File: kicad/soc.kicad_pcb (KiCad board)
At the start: 2 copper layers, 104.1 x 63.5 mm, 10 parts, among them J1 JACK_TRS_3PINS, J2 PS/2 Keyboard, J3 PS/2 Mouse, P1 LED MATRIX, P10 CODEC right, P11 CODEC inputs, P2 ALTERA_DE1_GPIO, P9 CODEC left, U2 DS3234

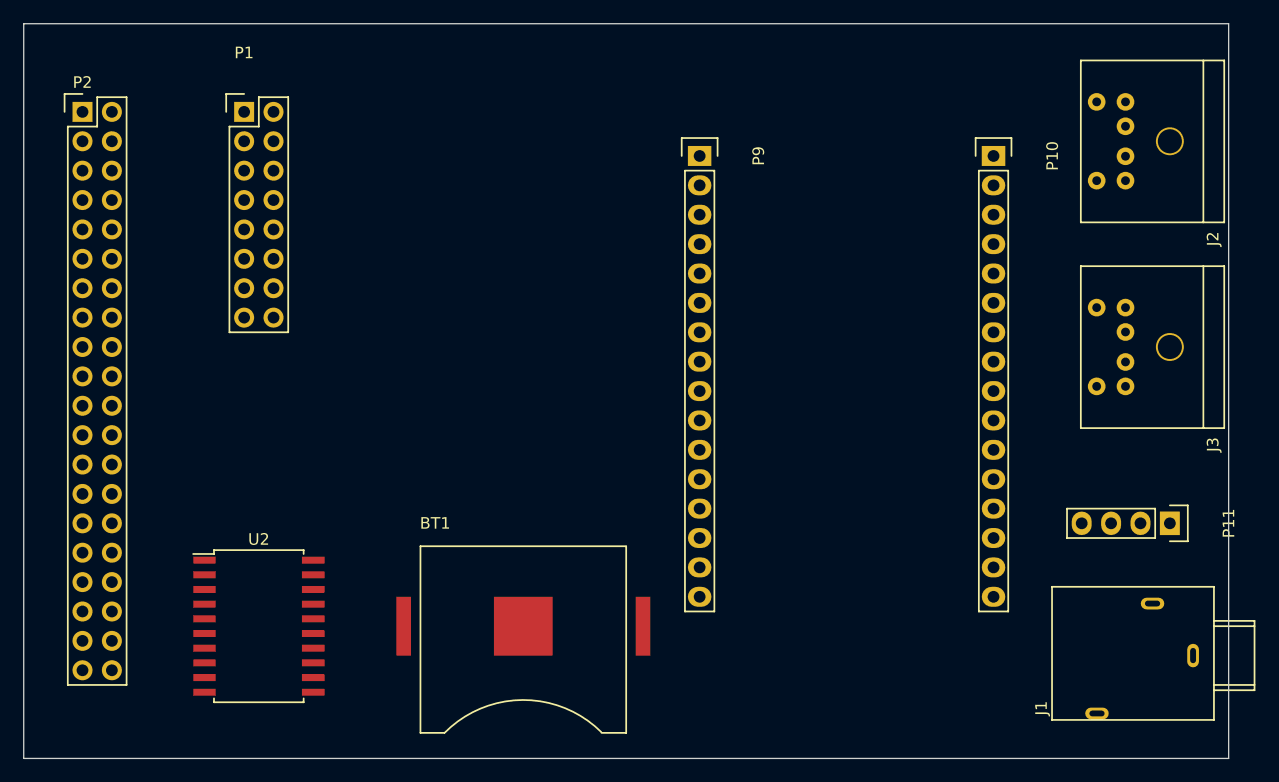
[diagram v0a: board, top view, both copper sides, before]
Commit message: close to final
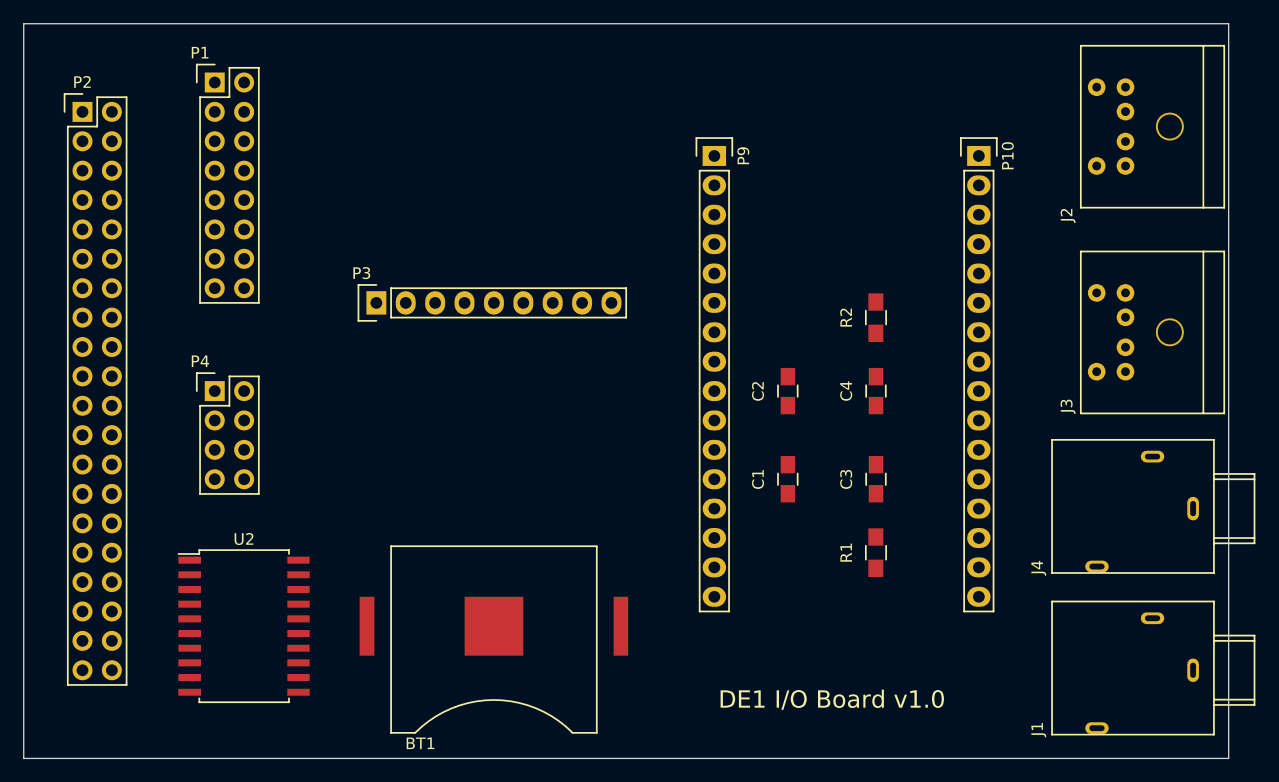
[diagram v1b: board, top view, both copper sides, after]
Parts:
- removed P11: CODEC inputs, Pin_Headers:Pin_Header_Straight_1x04
- added C1: 10nF, Capacitors_SMD:C_0805_HandSoldering, F.Cu at (106.7, 100.3)
- added C2: 10nF, Capacitors_SMD:C_0805_HandSoldering, F.Cu at (106.7, 92.7)
- added C3: 1uF, Capacitors_SMD:C_0805_HandSoldering, F.Cu at (114.3, 100.3)
- added C4: 1uF, Capacitors_SMD:C_0805_HandSoldering, F.Cu at (114.3, 92.7)
- added J4: Line In, mstock-pretty:SJI-3513N, F.Cu at (143.5, 102.9)
- added P3: Bluetooth, Socket_Strips:Socket_Strip_Straight_1x09, F.Cu at (71.1, 85.1)
- added P4: CONN_01X08, Pin_Headers:Pin_Header_Straight_2x04, F.Cu at (57.1, 92.7)
- added R1: 470, Resistors_SMD:R_0805_HandSoldering, F.Cu at (114.3, 106.7)
- added R2: 470, Resistors_SMD:R_0805_HandSoldering, F.Cu at (114.3, 86.4)
- J1: value JACK_TRS_3PINS -> Line Out
- moved P1 3.59 mm to (57.1, 66.0)
- moved BT1 2.54 mm to (81.3, 113.0)
- moved J1 1.27 mm to (143.5, 116.8)
- moved J2 1.27 mm to (139.7, 69.8)
- moved J3 1.27 mm to (139.7, 87.6)
- moved U2 1.27 mm to (59.7, 113.0)
- moved P10 1.27 mm to (123.2, 72.4)
- moved P9 1.27 mm to (100.3, 72.4)
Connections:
- net Net-(J1-Pad2) renamed /L_OUT
- net Net-(J1-Pad3) renamed /R_OUT
- J1 pad 1: Net-(J1-Pad1) -> GNDA
- J2 pad 2: (no net) -> Net-(J2-Pad2)
- J2 pad 6: (no net) -> Net-(J2-Pad6)
- J3 pad 2: (no net) -> Net-(J3-Pad2)
- J3 pad 6: (no net) -> Net-(J3-Pad6)
- P1 pad 12: (no net) -> Net-(P1-Pad12)
- P10 pad 1: (no net) -> Net-(P10-Pad1)
- P10 pad 10: (no net) -> Net-(P10-Pad10)
- P10 pad 11: (no net) -> Net-(P10-Pad11)
- P10 pad 12: (no net) -> Net-(P10-Pad12)
- P10 pad 13: Net-(P10-Pad13) -> GNDA
- P10 pad 15: Net-(P10-Pad15) -> /L_IN
- P10 pad 16: Net-(P10-Pad16) -> /R_IN
- P10 pad 2: (no net) -> Net-(P10-Pad2)
- P10 pad 3: (no net) -> Net-(P10-Pad3)
- P10 pad 4: (no net) -> Net-(P10-Pad4)
- P10 pad 5: (no net) -> Net-(P10-Pad5)
- P10 pad 6: (no net) -> Net-(P10-Pad6)
- P10 pad 7: (no net) -> Net-(P10-Pad7)
- P10 pad 8: (no net) -> Net-(P10-Pad8)
- P10 pad 9: (no net) -> Net-(P10-Pad9)
- P2 pad 1: (no net) -> /Serial1
- P2 pad 20: (no net) -> /IO_17
- P2 pad 21: (no net) -> /~BLE_CS
- P2 pad 22: (no net) -> /IO_19
- P2 pad 23: (no net) -> /IO_20
- P2 pad 24: (no net) -> /BLE_IRQ
- P2 pad 35: (no net) -> /IO_30
- P2 pad 36: (no net) -> /IO_31
- P2 pad 37: (no net) -> /IO_32
- P9 pad 13: Net-(J1-Pad1) -> GNDA
- P9 pad 14: Net-(J1-Pad1) -> GNDA
- P9 pad 2: (no net) -> Net-(P9-Pad2)
- P9 pad 9: (no net) -> Net-(P9-Pad9)
- U2 pad 10: (no net) -> Net-(U2-Pad10)
- U2 pad 11: (no net) -> Net-(U2-Pad11)
- U2 pad 12: (no net) -> Net-(U2-Pad12)
- U2 pad 13: (no net) -> Net-(U2-Pad13)
- U2 pad 14: (no net) -> Net-(U2-Pad14)
- U2 pad 2: (no net) -> Net-(U2-Pad2)
- U2 pad 3: (no net) -> Net-(U2-Pad3)
- U2 pad 5: (no net) -> Net-(U2-Pad5)
- U2 pad 6: (no net) -> Net-(U2-Pad6)
- U2 pad 7: (no net) -> Net-(U2-Pad7)
- U2 pad 8: (no net) -> Net-(U2-Pad8)
- U2 pad 9: (no net) -> Net-(U2-Pad9)
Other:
- board text added: "Bexkat Systems LLC 2016 www.bexkat.com"
- board text added: "DE1 I/O Board v1.0"
